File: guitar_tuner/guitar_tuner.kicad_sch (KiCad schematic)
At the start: 8 parts, among them SW1 Reset, SW2 Boot, U1 ESP32-S2-SOLO

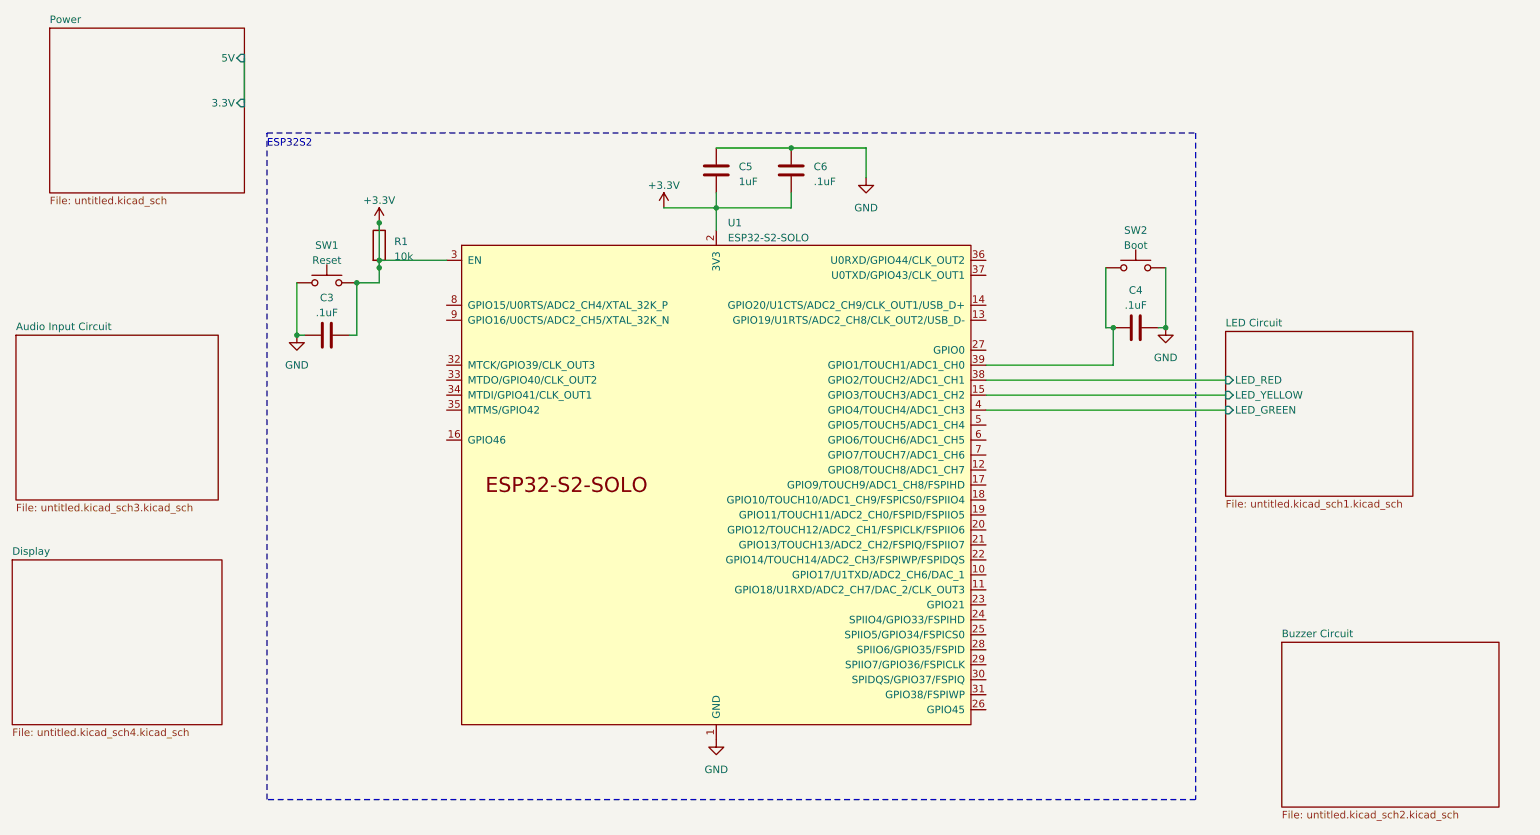
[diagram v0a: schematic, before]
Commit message: OLED
Addition of OLED Screen
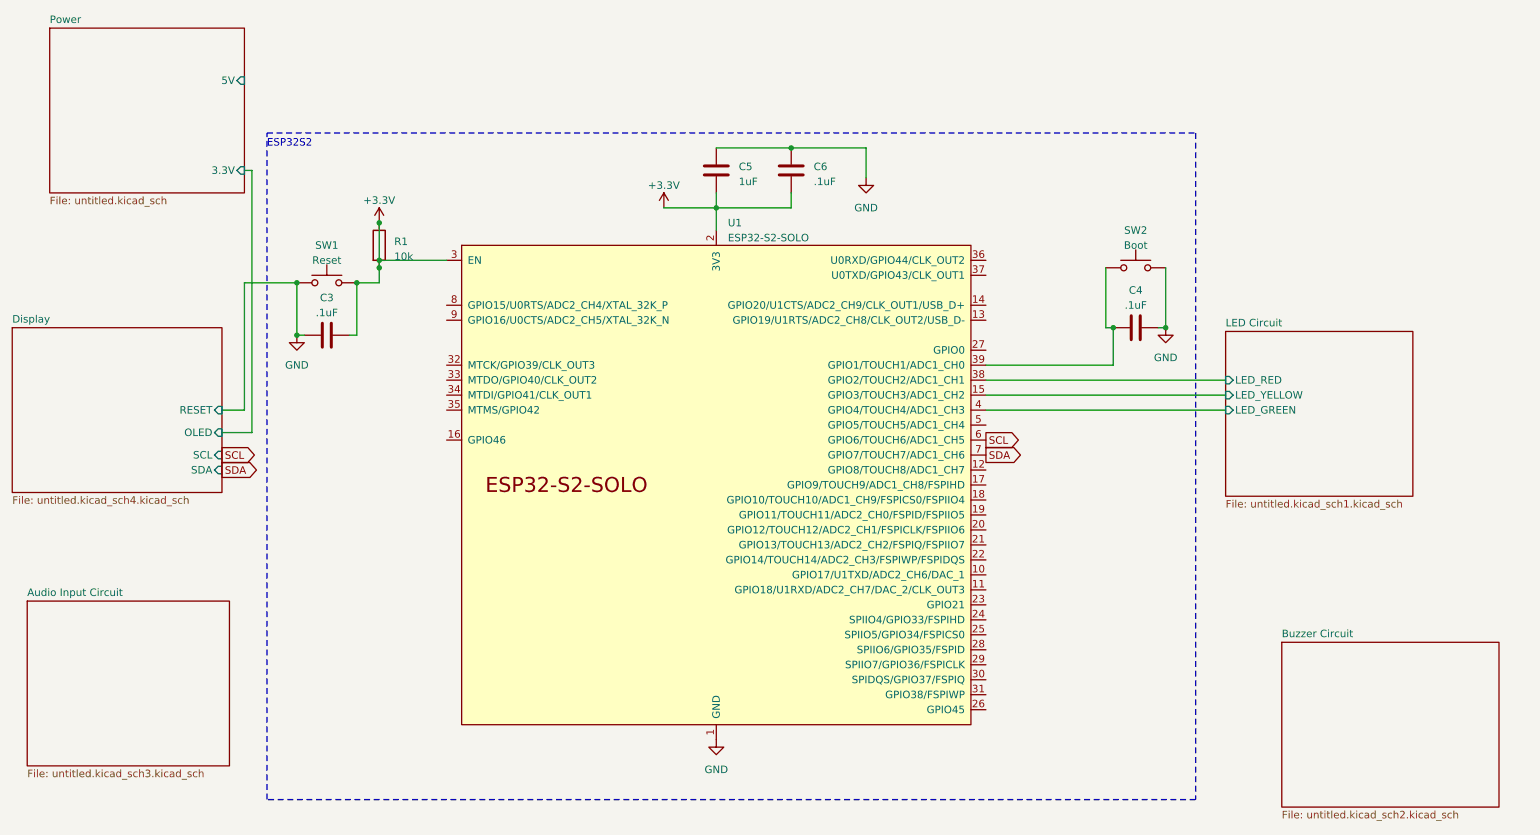
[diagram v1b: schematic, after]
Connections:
- net SCL: now reaches U1.6 (GPIO6/TOUCH6/ADC1_CH5)
- net SDA: now reaches U1.7 (GPIO7/TOUCH7/ADC1_CH6)
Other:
- sheet Display ports: added OLED, RESET, SCL, SDA; removed none
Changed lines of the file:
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@@
+	)
+	(junction
+		(at 66.04 66.04)
+		(diameter 0)
+		(color 0 0 0 0)
 	)
 	(junction
@@
 	(wire
 		(pts
+			(xy 57.15 87.63) (xy 57.15 66.04)
+		)
+		(stroke
+			(width 0)
+			(type default)
+		)
+	)
+	(wire
+		(pts
+			(xy 53.34 87.63) (xy 57.15 87.63)
+		)
+		(stroke
+			(width 0)
+			(type default)
+		)
+	)
+	(wire
+		(pts
 			(xy 76.2 66.04) (xy 76.2 74.93)
 		)
@@
 	(wire
 		(pts
+			(xy 57.15 66.04) (xy 66.04 66.04)
+		)
+		(stroke
+			(width 0)
+			(type default)
+		)
+	)
+	(wire
+		(pts
 			(xy 162.56 43.18) (xy 162.56 48.26)
 		)
@@
 	(wire
 		(pts
+			(xy 58.42 46.99) (xy 57.15 46.99)
+		)
+		(stroke
+			(width 0)
+			(type default)
+		)
+	)
+	(wire
+		(pts
 			(xy 137.16 53.34) (xy 137.16 57.15)
 		)
@@
 	(wire
 		(pts
+			(xy 53.34 91.44) (xy 58.42 91.44)
+		)
+		(stroke
+			(width 0)
+			(type default)
+		)
+	)
+	(wire
+		(pts
 			(xy 213.36 63.5) (xy 213.36 73.66)
 		)
@@
 	(wire
 		(pts
-			(xy 57.15 27.94) (xy 57.15 35.56)
+			(xy 58.42 91.44) (xy 58.42 46.99)
 		)
 		(stroke
@@
 			(width 0)
 			(type default)
+		)
+	)
+	(global_label "SCL"
+		(shape output)
+		(at 53.34 95.25 0)
+		(fields_autoplaced yes)
+		(effects
+			(font
+				(size 1.27 1.27)
+			)
+			(justify left)
+		)
+		(property "Intersheetrefs" "${INTERSHEET_REFS}"
+			(at 59.8328 95.25 0)
+			(effects
+				(font
+					(size 1.27 1.27)
+				)
+				(justify left)
+				(hide yes)
+			)
+		)
+	)
+	(global_label "SCL"
+		(shape output)
+		(at 182.88 92.71 0)
+		(fields_autoplaced yes)
+		(effects
+			(font
+				(size 1.27 1.27)
+			)
+			(justify left)
+		)
+		(property "Intersheetrefs" "${INTERSHEET_REFS}"
+			(at 189.3728 92.71 0)
+			(effects
+				(font
+					(size 1.27 1.27)
+				)
+				(justify left)
+				(hide yes)
+			)
+		)
+	)
+	(global_label "SDA"
+		(shape output)
+		(at 182.88 95.25 0)
+		(fields_autoplaced yes)
+		(effects
+			(font
+				(size 1.27 1.27)
+			)
+			(justify left)
+		)
+		(property "Intersheetrefs" "${INTERSHEET_REFS}"
+			(at 189.4333 95.25 0)
+			(effects
+				(font
+					(size 1.27 1.27)
+				)
+				(justify left)
+				(hide yes)
+			)
+		)
+	)
+	(global_label "SDA"
+		(shape output)
+		(at 53.34 97.79 0)
+		(fields_autoplaced yes)
+		(effects
+			(font
+				(size 1.27 1.27)
+			)
+			(justify left)
+		)
+		(property "Intersheetrefs" "${INTERSHEET_REFS}"
+			(at 59.8933 97.79 0)
+			(effects
+				(font
+					(size 1.27 1.27)
+				)
+				(justify left)
+				(hide yes)
+			)
 		)
 	)
@@
 	)
 	(sheet
-		(at 17.78 113.03)
+		(at 17.78 73.66)
 		(size 35.56 27.94)
 		(exclude_from_sim no)
@@
 		)
 		(property "Sheetname" "Display"
-			(at 17.78 112.3184 0)
+			(at 17.78 72.9484 0)
 			(effects
 				(font
@@
 		)
 		(property "Sheetfile" "untitled.kicad_sch4.kicad_sch"
-			(at 17.78 141.5546 0)
+			(at 17.78 102.1846 0)
 			(effects
 				(font
@@
 				)
 				(justify left top)
+			)
+		)
+		(pin "OLED" input
+			(at 53.34 91.44 0)
+			(effects
+				(font
+					(size 1.27 1.27)
+				)
+				(justify right)
+			)
+		)
+		(pin "RESET" input
+			(at 53.34 87.63 0)
+			(effects
+				(font
+					(size 1.27 1.27)
+				)
+				(justify right)
+			)
+		)
+		(pin "SCL" input
+			(at 53.34 95.25 0)
+			(effects
+				(font
+					(size 1.27 1.27)
+				)
+				(justify right)
+			)
+		)
+		(pin "SDA" input
+			(at 53.34 97.79 0)
+			(effects
+				(font
+					(size 1.27 1.27)
+				)
+				(justify right)
 			)
 		)
@@
 	)
 	(sheet
-		(at 18.415 74.93)
+		(at 20.32 120.015)
 		(size 34.29 27.94)
 		(exclude_from_sim no)
@@
 		)
 		(property "Sheetname" "Audio Input Circuit"
-			(at 18.415 74.2184 0)
+			(at 20.32 119.3034 0)
 			(effects
 				(font
@@
 		)
 		(property "Sheetfile" "untitled.kicad_sch3.kicad_sch"
-			(at 18.415 103.4546 0)
+			(at 20.32 148.5396 0)
 			(effects
 				(font
@@
 			)
 		)
+		(pin "3.3V" input
+			(at 57.15 46.99 0)
+			(effects
+				(font
+					(size 1.27 1.27)
+				)
+				(justify right)
+			)
+		)
 		(pin "5V" input
-			(at 57.15 27.94 0)
-			(effects
-				(font
-					(size 1.27 1.27)
-				)
-				(justify right)
-			)
-		)
-		(pin "3.3V" input
-			(at 57.15 35.56 0)
-			(effects
-				(font
+			(at 57.15 31.75 0)
+			(effects
+				(font
